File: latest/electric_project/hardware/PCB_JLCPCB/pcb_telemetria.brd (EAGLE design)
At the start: 108.1 x 122.7 mm, 47 parts

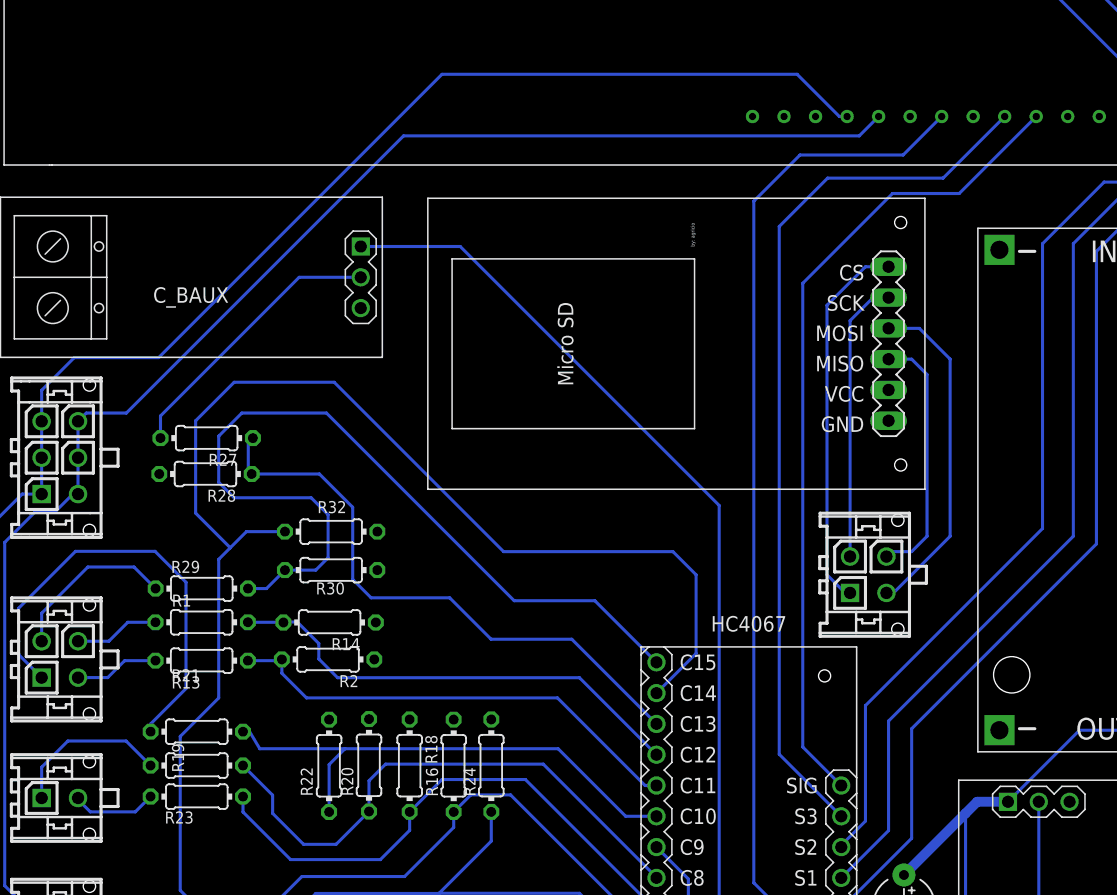
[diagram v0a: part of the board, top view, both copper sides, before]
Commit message: up
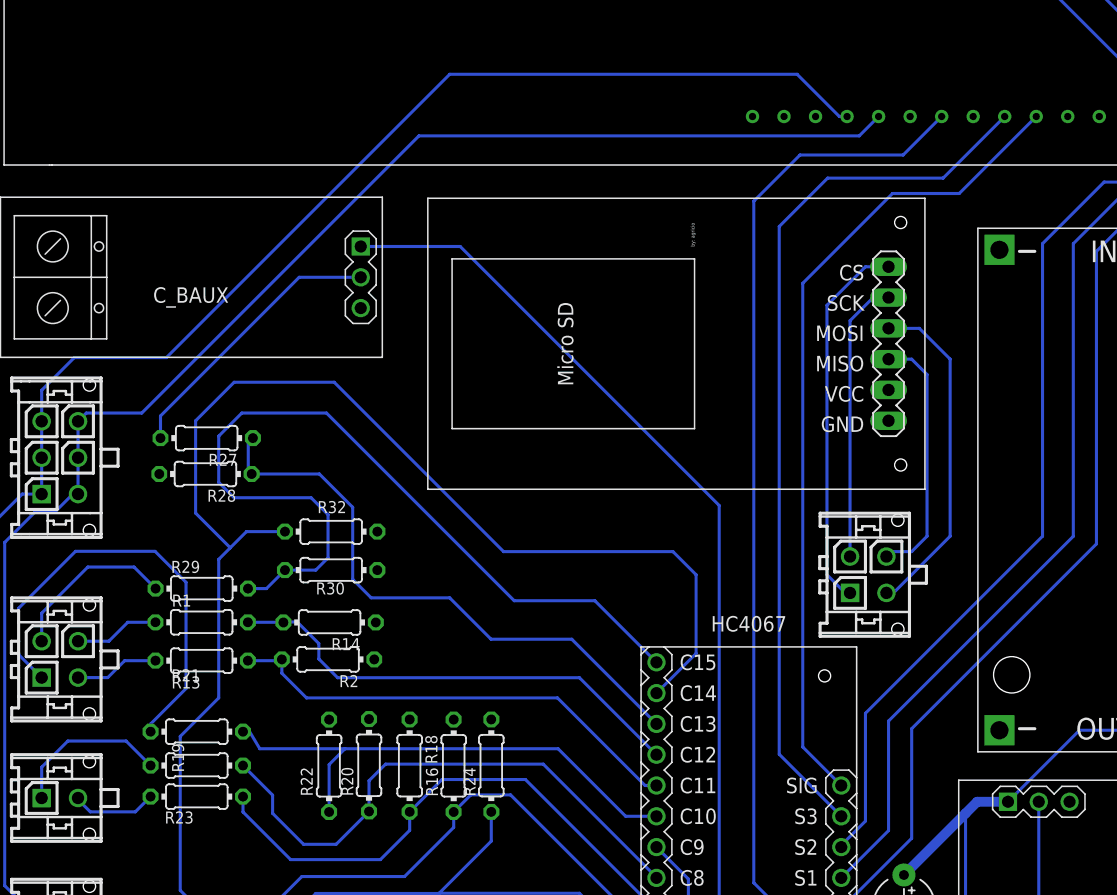
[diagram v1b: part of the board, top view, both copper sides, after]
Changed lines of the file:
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@@
 <?xml version="1.0" encoding="utf-8"?>
 <!DOCTYPE eagle SYSTEM "eagle.dtd">
-<eagle version="9.5.0">
+<eagle version="9.5.1">
 <drawing>
 <settings>
@@
 <wire x1="74.83855625" y1="22.621246875" x2="74.83855625" y2="22.76855625" width="0.254" layer="16"/>
 <wire x1="74.83855625" y1="22.76855625" x2="76.835" y2="24.765" width="0.254" layer="16"/>
-<wire x1="76.835" y1="24.765" x2="76.835" y2="34.29" width="0.254" layer="16"/>
-<wire x1="91.44" y1="48.895" x2="91.44" y2="72.39" width="0.254" layer="16"/>
+<wire x1="76.835" y1="24.765" x2="76.835" y2="33.655" width="0.254" layer="16"/>
+<wire x1="91.44" y1="48.26" x2="91.44" y2="72.39" width="0.254" layer="16"/>
 <wire x1="91.44" y1="72.39" x2="96.52" y2="77.47" width="0.254" layer="16"/>
 <wire x1="97.79" y1="77.47" x2="100.965" y2="80.645" width="0.254" layer="16"/>
@@
 <wire x1="78.74" y1="102.87" x2="75.31951875" y2="106.29048125" width="0.254" layer="16"/>
 <wire x1="75.31951875" y1="106.29048125" x2="75.31951875" y2="107.777559375" width="0.254" layer="16"/>
-<wire x1="76.835" y1="34.29" x2="91.44" y2="48.895" width="0.254" layer="16"/>
+<wire x1="76.835" y1="33.655" x2="91.44" y2="48.26" width="0.254" layer="16"/>
 <wire x1="96.52" y1="77.47" x2="97.79" y2="77.47" width="0.254" layer="16"/>
 <wire x1="100.965" y1="84.455" x2="82.55" y2="102.87" width="0.254" layer="16"/>
@@
 <vertex x="-5.715" y="116.205"/>
 </polygon>
+<wire x1="80.51951875" y1="82.877559375" x2="70.11951875" y2="107.777559375" width="0" layer="19" extent="1-1"/>
+<wire x1="87.884" y1="71.882" x2="80.51951875" y2="82.877559375" width="0" layer="19" extent="1-1"/>
+<wire x1="87.884" y1="32.258" x2="87.884" y2="71.882" width="0" layer="19" extent="1-1"/>
+<wire x1="93.670121875" y1="26.360109375" x2="87.884" y2="32.258" width="0" layer="19" extent="1-1"/>
+<wire x1="100.838" y1="27.305" x2="93.670121875" y2="26.360109375" width="0" layer="19" extent="1-1"/>
+<wire x1="102.362" y1="20.701" x2="100.838" y2="27.305" width="0" layer="19" extent="1-1"/>
+<wire x1="80.01" y1="15.24" x2="93.670121875" y2="26.360109375" width="0" layer="19" extent="1-1"/>
+<wire x1="74.83855625" y1="15.001246875" x2="80.01" y2="15.24" width="0" layer="19" extent="1-1"/>
+<wire x1="74.83855625" y1="9.921246875" x2="74.83855625" y2="15.001246875" width="0" layer="19" extent="1-1"/>
+<wire x1="80.01" y1="6.985" x2="74.83855625" y2="9.921246875" width="0" layer="19" extent="1-1"/>
+<wire x1="51.7906" y1="2.778759375" x2="74.83855625" y2="9.921246875" width="0" layer="19" extent="1-1"/>
+<wire x1="47.752" y1="16.728446875" x2="51.7906" y2="2.778759375" width="0" layer="19" extent="1-1"/>
+<wire x1="43.942" y1="16.728446875" x2="47.752" y2="16.728446875" width="0" layer="19" extent="1-1"/>
+<wire x1="40.132" y1="16.728446875" x2="43.942" y2="16.728446875" width="0" layer="19" extent="1-1"/>
+<wire x1="36.322" y1="16.728446875" x2="40.132" y2="16.728446875" width="0" layer="19" extent="1-1"/>
+<wire x1="32.512" y1="16.728446875" x2="36.322" y2="16.728446875" width="0" layer="19" extent="1-1"/>
+<wire x1="32.5983625" y1="33.13684375" x2="32.512" y2="16.728446875" width="0" layer="19" extent="1-1"/>
+<wire x1="35.89020625" y1="33.177484375" x2="32.5983625" y2="33.13684375" width="0" layer="19" extent="1-1"/>
+<wire x1="39.243" y1="33.147" x2="35.89020625" y2="33.177484375" width="0" layer="19" extent="1-1"/>
+<wire x1="42.87520625" y1="33.13684375" x2="39.243" y2="33.147" width="0" layer="19" extent="1-1"/>
+<wire x1="36.322" y1="38.1" x2="35.89020625" y2="33.177484375" width="0" layer="19" extent="1-1"/>
+<wire x1="36.449" y1="41.148" x2="36.322" y2="38.1" width="0" layer="19" extent="1-1"/>
+<wire x1="36.576" y1="45.466" x2="36.449" y2="41.148" width="0" layer="19" extent="1-1"/>
+<wire x1="36.576" y1="48.641" x2="36.576" y2="45.466" width="0" layer="19" extent="1-1"/>
+<wire x1="35.209478125" y1="67.076315625" x2="36.576" y2="48.641" width="0" layer="19" extent="1-1"/>
+<wire x1="18.590259375" y1="53.393340625" x2="36.576" y2="48.641" width="0" layer="19" extent="1-1"/>
 </signal>
 <signal name="22">
 <contactref element="U$1" pad="22"/>
-<wire x1="15.875" y1="58.42" x2="38.735" y2="81.28" width="0.254" layer="16"/>
+<wire x1="17.145" y1="58.42" x2="40.005" y2="81.28" width="0.254" layer="16"/>
 <wire x1="76.321946875" y1="81.2799875" x2="77.91951875" y2="82.877559375" width="0.254" layer="16"/>
-<wire x1="76.321946875" y1="81.2799875" x2="38.735" y2="81.28" width="0.254" layer="16"/>
+<wire x1="76.321946875" y1="81.2799875" x2="40.005" y2="81.28" width="0.254" layer="16"/>
 <contactref element="X5" pad="P$5"/>
 <contactref element="X5" pad="P$6"/>
 <contactref element="X5" pad="P$4"/>
 <wire x1="11.89" y1="51.737" x2="11.89" y2="52.07" width="0.254" layer="16"/>
-<wire x1="11.89" y1="52.07" x2="11.89" y2="54.61" width="0.254" layer="16"/>
+<wire x1="11.89" y1="52.07" x2="11.89" y2="54.737" width="0.254" layer="16"/>
 <wire x1="11.89" y1="54.737" x2="11.89" y2="57.737" width="0.254" layer="16"/>
 <wire x1="11.89" y1="57.737" x2="12.573" y2="58.42" width="0.254" layer="16"/>
-<wire x1="12.573" y1="58.42" x2="15.875" y2="58.42" width="0.254" layer="16"/>
+<wire x1="12.573" y1="58.42" x2="17.145" y2="58.42" width="0.254" layer="16"/>
 <contactref element="X1" pad="P$6"/>
 <wire x1="8.89" y1="16.39" x2="8.83" y2="16.45" width="0.254" layer="16"/>
@@
 <wire x1="8.89" y1="13.39" x2="8.83" y2="13.45" width="0.254" layer="16"/>
 <wire x1="8.83" y1="13.45" x2="8.83" y2="16.45" width="0.254" layer="16"/>
-<wire x1="11.89" y1="54.737" x2="11.89" y2="54.61" width="0.254" layer="16"/>
 </signal>
 <signal name="21">
 <contactref element="U$1" pad="21"/>
-<wire x1="71.202103125" y1="86.359975" x2="41.91" y2="86.36" width="0.254" layer="16"/>
+<wire x1="71.202103125" y1="86.359975" x2="42.545" y2="86.36" width="0.254" layer="16"/>
 <wire x1="8.8782" y1="60.2888" x2="11.5814" y2="62.992" width="0.254" layer="16"/>
-<wire x1="11.5814" y1="62.992" x2="18.542" y2="62.992" width="0.254" layer="16"/>
-<wire x1="18.542" y1="62.992" x2="41.91" y2="86.36" width="0.254" layer="16"/>
+<wire x1="11.5814" y1="62.992" x2="19.177" y2="62.992" width="0.254" layer="16"/>
+<wire x1="19.177" y1="62.992" x2="42.545" y2="86.36" width="0.254" layer="16"/>
 <contactref element="X5" pad="P$2"/>
 <contactref element="X5" pad="P$1"/>
